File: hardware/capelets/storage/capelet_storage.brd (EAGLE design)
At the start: 16.5 x 12.7 mm, 4 parts

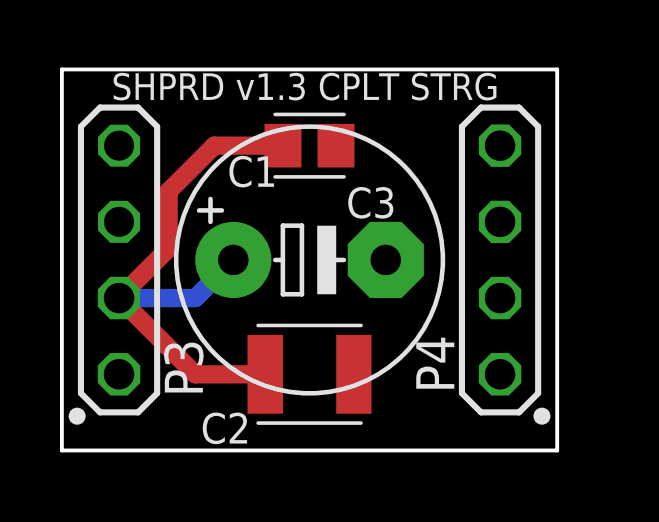
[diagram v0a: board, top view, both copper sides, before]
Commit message: hardware: updated capelets
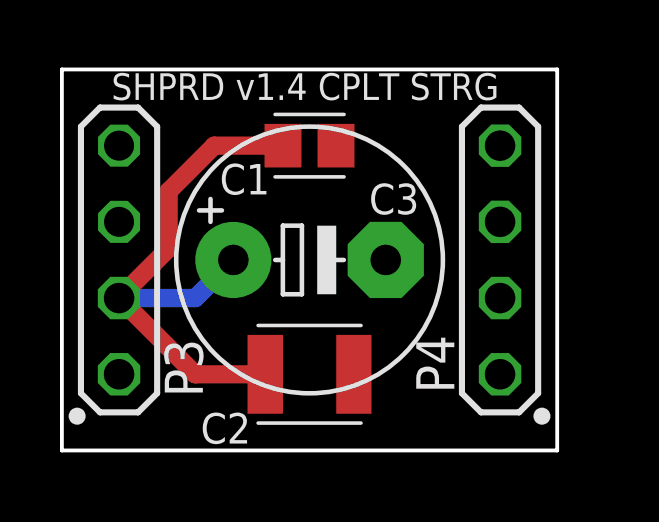
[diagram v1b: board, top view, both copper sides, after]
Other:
- board text added: "SHPRD v1.4 CPLT STRG"
- board text removed: "SHPRD v1.3 CPLT STRG"
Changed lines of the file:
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@@
 <dimension x1="17.145" y1="12.7" x2="17.145" y2="0" x3="20.32" y3="6.35" textsize="1.143" textratio="16" layer="47"/>
 <dimension x1="0.635" y1="12.7" x2="17.145" y2="12.7" x3="8.89" y3="13.97" textsize="1.143" textratio="16" layer="47"/>
-<text x="2.286" y="11.684" size="0.889" layer="25" font="vector" ratio="16">SHPRD v1.3 CPLT STRG</text>
+<text x="2.286" y="11.684" size="0.889" layer="25" font="vector" ratio="16">SHPRD v1.4 CPLT STRG</text>
 </plain>
 <attributes>
@@
 <element name="U$1" library="shepherd" package="SHPRD_CPLT_S" value="SHPRD_CPLT_S" x="0" y="0" smashed="yes"/>
 <element name="C1" library="shepherd" package="CAPC2012X145" package3d_urn="urn:adsk.eagle:package:4930364/1" value="" x="8.89" y="10.16" smashed="yes">
-<attribute name="NAME" x="6.985" y="8.7876" size="1.016" layer="25" font="vector" ratio="16" align="bottom-center"/>
+<attribute name="NAME" x="6.731" y="8.5336" size="1.016" layer="25" font="vector" ratio="16" align="bottom-center"/>
 <attribute name="VALUE" x="8.89" y="8.4844" size="1.27" layer="27" align="top-center"/>
 </element>
@@
 </element>
 <element name="C3" library="rcl" library_urn="urn:adsk.eagle:library:334" package="E5-8,5" package3d_urn="urn:adsk.eagle:package:23374/1" value="" x="8.89" y="6.35" smashed="yes">
-<attribute name="NAME" x="10.1092" y="7.747" size="1.016" layer="25" font="vector" ratio="16"/>
+<attribute name="NAME" x="10.8712" y="7.874" size="1.016" layer="25" font="vector" ratio="16"/>
 <attribute name="SPICEPREFIX" value="C" x="8.89" y="6.35" size="1.778" layer="27" display="off"/>
 <attribute name="VALUE" x="6.3754" y="3.3274" size="1.27" layer="27" ratio="10"/>
